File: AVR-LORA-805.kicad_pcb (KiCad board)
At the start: 2 copper layers, 51.7 x 29.2 mm, 39 parts, among them J1 Batt, J2 Solar, J3 SMA, J4 CONN_01X14, J5 CONN_01X14, U1 MCP1700-3302E_SOT23, U2 RFM95HW, U3 AVR128DB28, Y1 24MHz, Y2 32768Hz

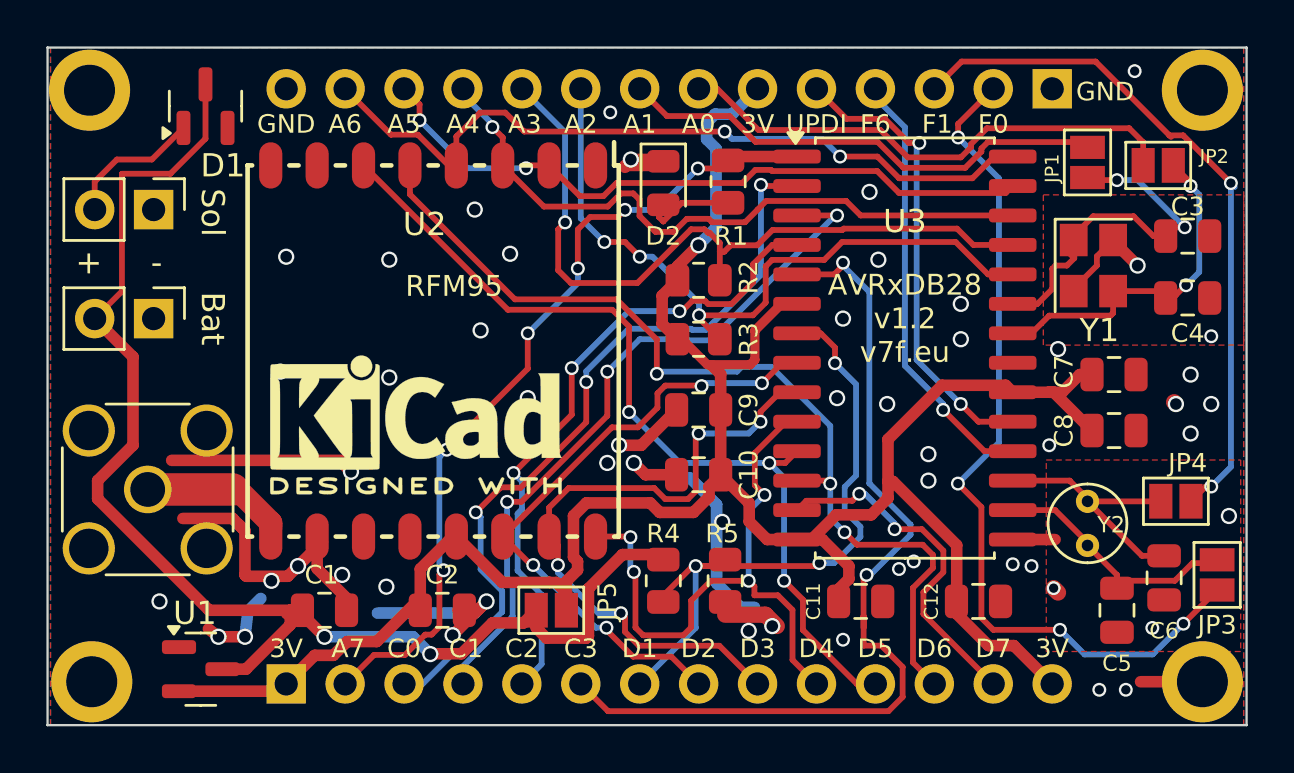
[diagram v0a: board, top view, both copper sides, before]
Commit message: Minor cleanups AVR 805 version
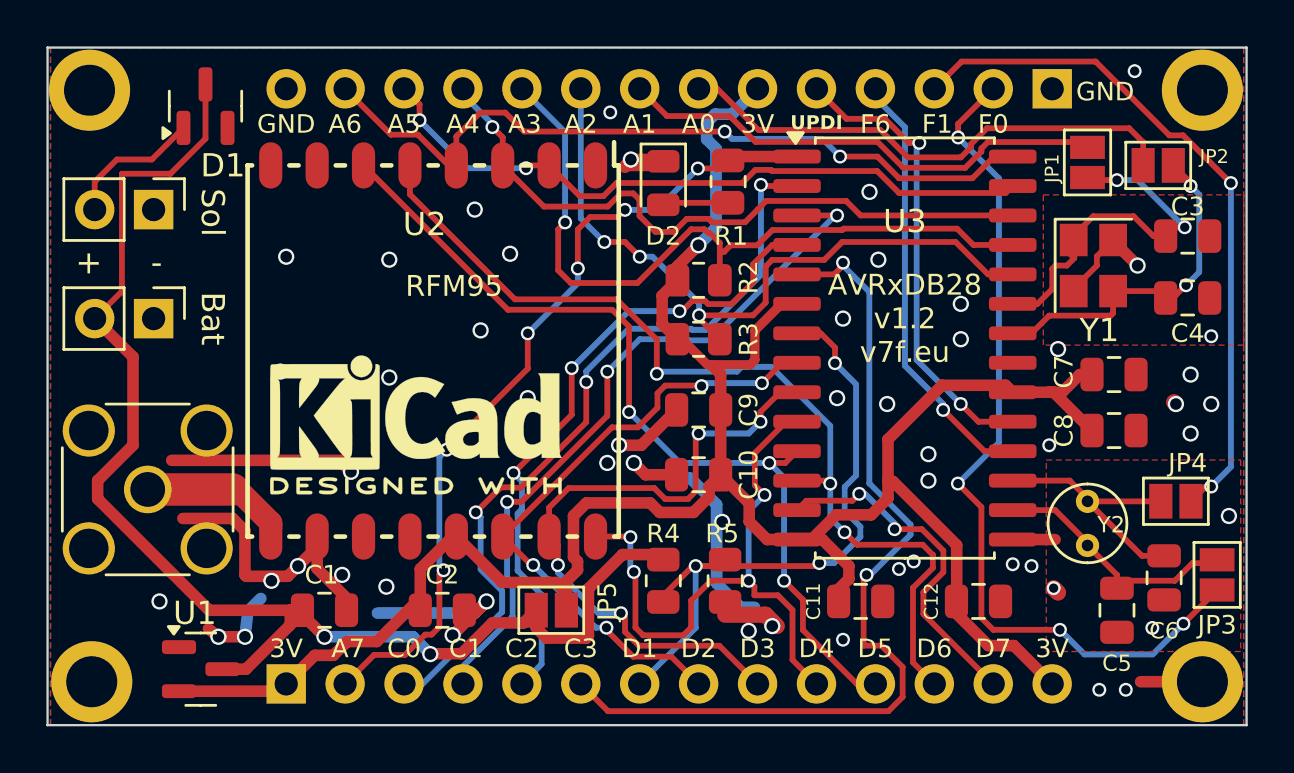
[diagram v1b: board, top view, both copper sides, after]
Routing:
- net Net-(D2-A): track 4.00 -> 2.83 mm
- net GND: track 60.4 -> 59.7 mm
- net /A0: track 15.3 -> 14.7 mm
- net /C3: track 39.1 -> 38.6 mm
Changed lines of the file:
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@@
 			(net 37 "unconnected-(D1-K-Pad2)")
 			(pinfunction "K")
-			(pintype "passive")
+			(pintype "passive+no_connect")
 		)
 		(pad "3" smd roundrect
@@
 	)
 	(gr_text "UPDI"
-		(at 100.838 84.963 0)
+		(at 100.838 84.9 0)
 		(layer "F.SilkS")
 		(effects
 			(font
-				(size 0.8 0.8)
-				(thickness 0.15)
+				(size 0.6 0.6)
+				(thickness 0.1)
+				(bold yes)
 			)
 		)
@@
 	)
 	(gr_text "D4"
-		(at 100.838 107.188 180)
+		(at 100.838 107.1 180)
 		(layer "B.SilkS")
 		(effects
@@
 	)
 	(segment
-		(start 95.037 88.354)
-		(end 97.028 88.354)
-		(width 0.25)
-		(layer "F.Cu")
-		(net 1)
-	)
-	(segment
-		(start 94.234 89.157)
-		(end 94.237 89.157)
-		(width 0.25)
-		(layer "F.Cu")
-		(net 1)
-	)
-	(segment
-		(start 94.043032 88.631468)
+		(start 94.3205 88.354)
 		(end 94.234 88.4405)
 		(width 0.25)
@@
 	)
 	(segment
-		(start 94.234 89.157)
-		(end 94.043032 88.966032)
+		(start 97.028 88.354)
+		(end 94.3205 88.354)
 		(width 0.25)
 		(layer "F.Cu")
@@
 	)
 	(segment
-		(start 94.043032 88.966032)
-		(end 94.043032 88.631468)
-		(width 0.25)
-		(layer "F.Cu")
-		(net 1)
-	)
-	(segment
-		(start 94.234 89.157)
-		(end 95.037 88.354)
-		(width 0.25)
-		(layer "F.Cu")
-		(net 1)
-	)
-	(segment
-		(start 77.184 102.87)
-		(end 77.313 102.741)
-		(width 0.25)
-		(layer "F.Cu")
-		(net 2)
-	)
-	(segment
 		(start 75.678 100.711)
 		(end 72.009 100.711)
@@
 	)
 	(segment
-		(start 76.2 102.489)
-		(end 76.1365 102.4255)
-		(width 0.5)
-		(layer "F.Cu")
-		(net 4)
-	)
-	(segment
 		(start 94.234 86.484)
 		(end 92.922959 86.484)
@@
 	)
 	(segment
-		(start 75.692 101.981)
-		(end 76.1365 102.4255)
-		(width 0.5)
-		(layer "F.Cu")
-		(net 4)
-	)
-	(segment
 		(start 80.579 105.393)
 		(end 80.579 105.918)
@@
 	)
 	(segment
-		(start 76.1365 102.4255)
-		(end 75.946 102.235)
+		(start 75.692 101.981)
+		(end 76.2 102.489)
 		(width 0.5)
 		(layer "F.Cu")
@@
 	)
 	(segment
-		(start 111.926 91.759)
-		(end 111.926 92.159)
-		(width 0.25)
-		(layer "F.Cu")
-		(net 4)
-	)
-	(segment
 		(start 78.045393 104.453607)
 		(end 76.259607 104.453607)
@@
 	)
 	(segment
-		(start 78.154 105.918)
-		(end 78.0025 106.0695)
-		(width 0.5)
-		(layer "F.Cu")
-		(net 5)
-	)
-	(segment
 		(start 71.374 98.806)
 		(end 71.374 94.996)
@@
 	)
 	(segment
-		(start 69.849002 93.345)
-		(end 69.723 93.345)
-		(width 0.25)
-		(layer "F.Cu")
-		(net 5)
-	)
-	(segment
 		(start 70.898001 87.101999)
 		(end 72.987823 87.101999)
@@
 	)
 	(segment
-		(start 109.298 93.98)
-		(end 108.871232 93.98)
-		(width 0.25)
-		(layer "F.Cu")
-		(net 9)
-	)
-	(segment
-		(start 113.626 92.344002)
-		(end 113.626 92.159)
-		(width 0.25)
-		(layer "F.Cu")
-		(net 9)
-	)
-	(segment
 		(start 116.205 92.456)
 		(end 116.332 92.329)
@@
 	)
 	(segment
-		(start 112.537 87.376)
-		(end 112.522 87.391)
-		(width 0.25)
-		(layer "F.Cu")
-		(net 10)
-	)
-	(segment
 		(start 112.765999 88.933999)
 		(end 114.509999 88.933999)
@@
 	)
 	(segment
-		(start 101.727002 89.026998)
-		(end 101.727002 88.9)
-		(width 0.25)
-		(layer "B.Cu")
-		(net 16)
-	)
-	(segment
-		(start 85.598 109.093)
-		(end 85.679001 109.011999)
-		(width 0.25)
-		(layer "B.Cu")
-		(net 16)
-	)
-	(segment
 		(start 93.218 94.234)
 		(end 91.821 95.631)
@@
 	)
 	(segment
-		(start 102.86799 106.6794)
-		(end 102.86799 106.17401)
-		(width 0.25)
-		(layer "F.Cu")
-		(net 18)
-	)
-	(segment
 		(start 91.853001 110.268001)
 		(end 103.942001 110.268001)
@@
 	)
 	(segment
-		(start 103.378 109.093)
-		(end 103.03581 109.093)
-		(width 0.25)
-		(layer "F.Cu")
-		(net 23)
-	)
-	(segment
 		(start 100.253998 106.769996)
 		(end 100.253998 105.460998)
@@
 	)
 	(segment
-		(start 87.212996 86.741)
-		(end 87.313 86.741)
-		(width 0.25)
-		(layer "F.Cu")
-		(net 28)
-	)
-	(segment
 		(start 91.84113 88.516021)
 		(end 89.088021 88.516021)
@@
 	)
 	(segment
-		(start 96.6705 91.694)
-		(end 96.77441 91.694)
-		(width 0.25)
-		(layer "F.Cu")
-		(net 29)
-	)
-	(segment
 		(start 96.6705 90.464498)
 		(end 96.860502 90.464498)
@@
 	)
 	(segment
-		(start 116.0535 85.4465)
-		(end 116.121001 85.514001)
-		(width 0.25)
-		(layer "F.Cu")
-		(net 35)
-	)
-	(segment
 		(start 116.6465 85.4465)
 		(end 116.0535 85.4465)
@@
 		(net 35)
 	)
-	(segment
-		(start 118.703 87.503)
-		(end 118.872 87.672)
-		(width 0.25)
-		(layer "B.Cu")
-		(net 35)
-	)
